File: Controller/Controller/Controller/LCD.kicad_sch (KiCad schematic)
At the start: 49 parts, among them J8 Conn_01x06_MountingPin, J9 Conn_01x50_MountingPin, U10 LTC1261L, U12 LM2931-ADJ_soic-8, U5 BD00C0AWFP, U6 LMR50410, U8 C85037, U9 BD00C0AWFP

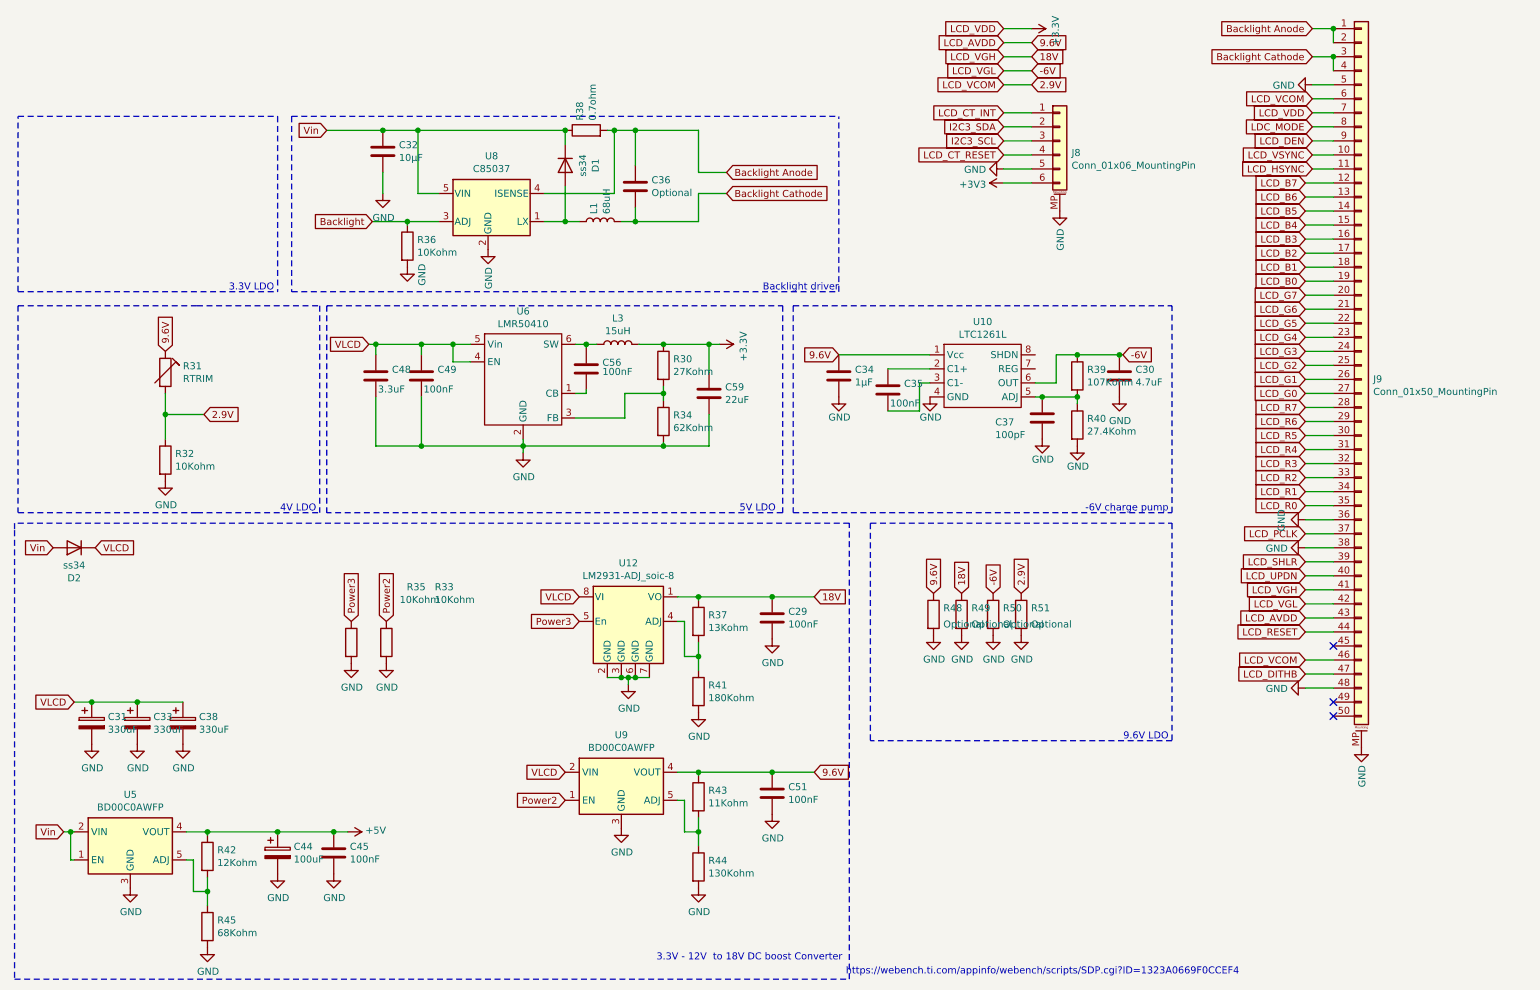
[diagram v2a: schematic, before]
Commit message: Final Version Tested
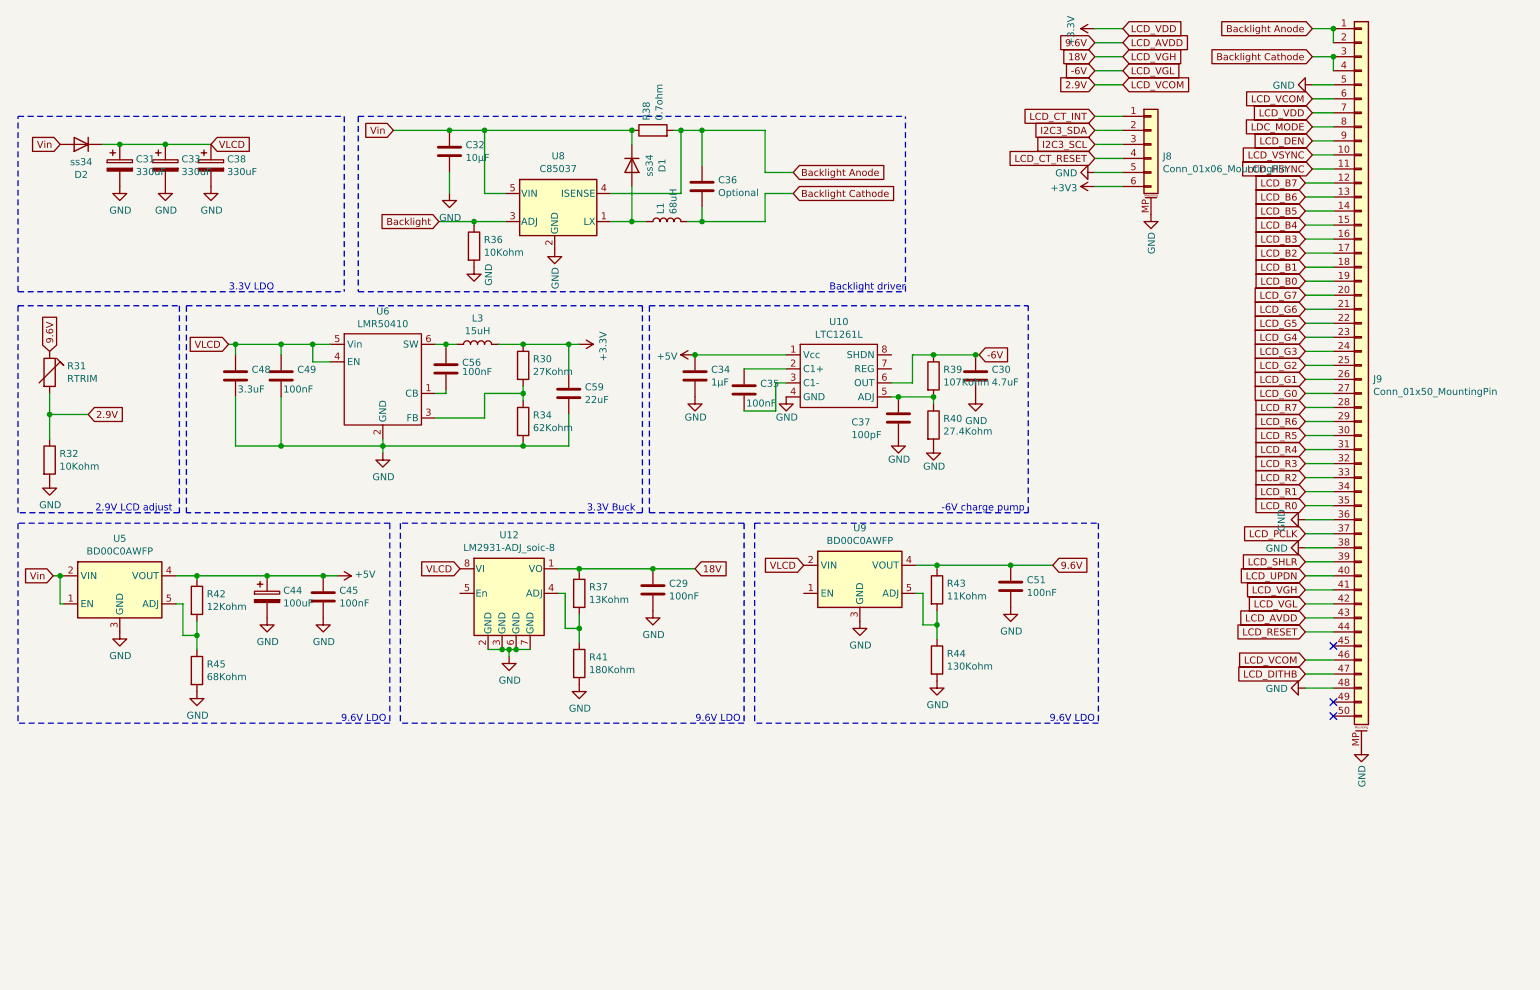
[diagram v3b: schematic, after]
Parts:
- removed R33, R35: 10Kohm, Resistor_SMD:R_0805_2012Metric_Pad1.20x1.40mm_HandSolder, symbol Device:R
- removed R48, R49, R50, R51: Optional, Resistor_SMD:R_0805_2012Metric_Pad1.20x1.40mm_HandSolder, symbol Device:R
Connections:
- net +5V: now also C34.1, U10.1 (Vcc)
- net 9.6V: no longer C34.1, U10.1 (Vcc)
- net Power2: no longer names the net of U9.1 (EN)
- net Power3: no longer names the net of U12.5 (En)
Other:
- note added: "2.9V LCD adjust"
- note added: "3.3V Buck"
- note removed: "3.3V - 12V to 18V DC boost Converter"
- note removed: "4V LDO"
- note removed: "5V LDO"
- note removed: "https://webench.ti.com/appinfo/webench/scripts/SDP.cgi?ID=1323A0669F0CCEF4"
- moved on the sheet: C29, C30, C31, C32, C33, C34, C35, C36, C37, C38, C44, C45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
